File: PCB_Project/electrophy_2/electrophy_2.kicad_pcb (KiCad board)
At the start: 4 copper layers, 35 x 35 mm, 47 parts, among them IC1 ESP32-C3FN4, J1 USB_C_Receptacle_USB2.0_14P, J3 Conn_01x04, U1 LSM6DSV320XTR, U2 BQ21040DBV, U3 TPS27081ADDCR, U4 USBLC6-2SC6, U5 MIC5504-3.3YM5, Y1 40MHZ 15pf, Y2 32 KHz

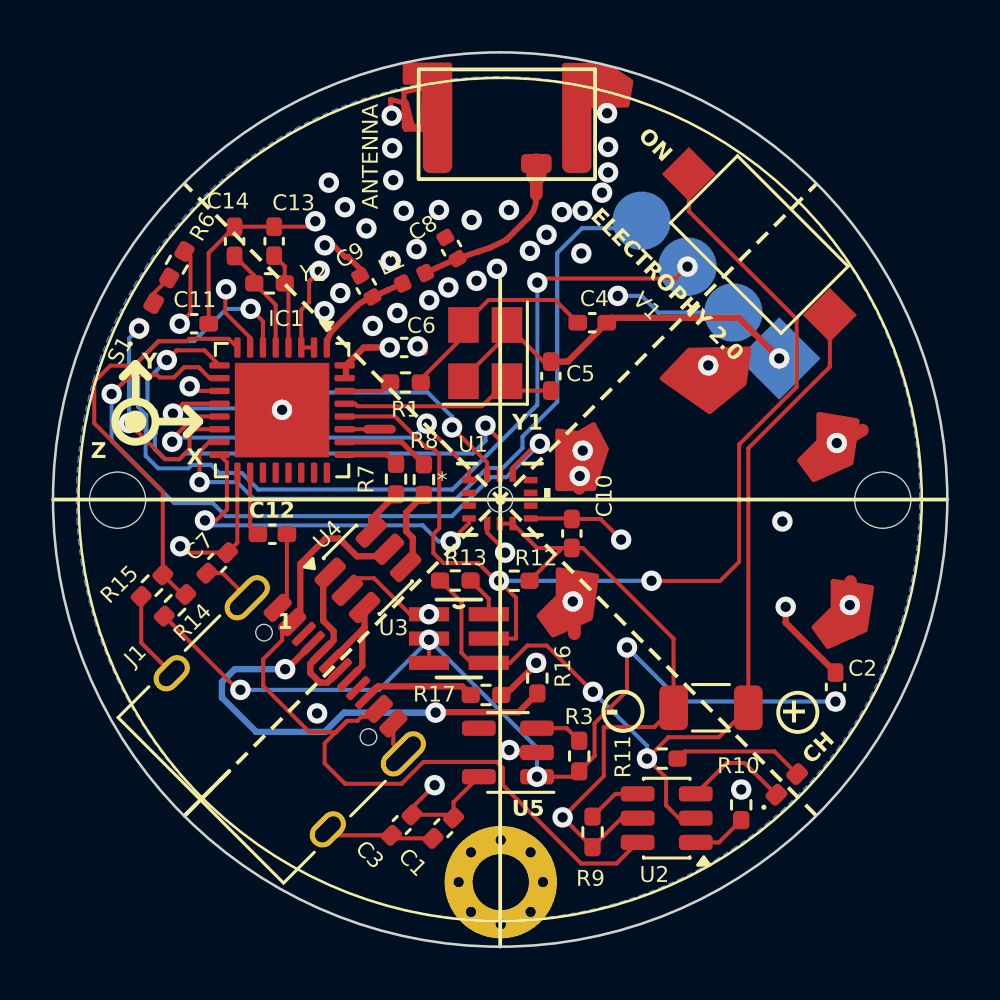
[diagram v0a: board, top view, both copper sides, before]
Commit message: order placed for ElectroPhy 2.0 V1 PCB
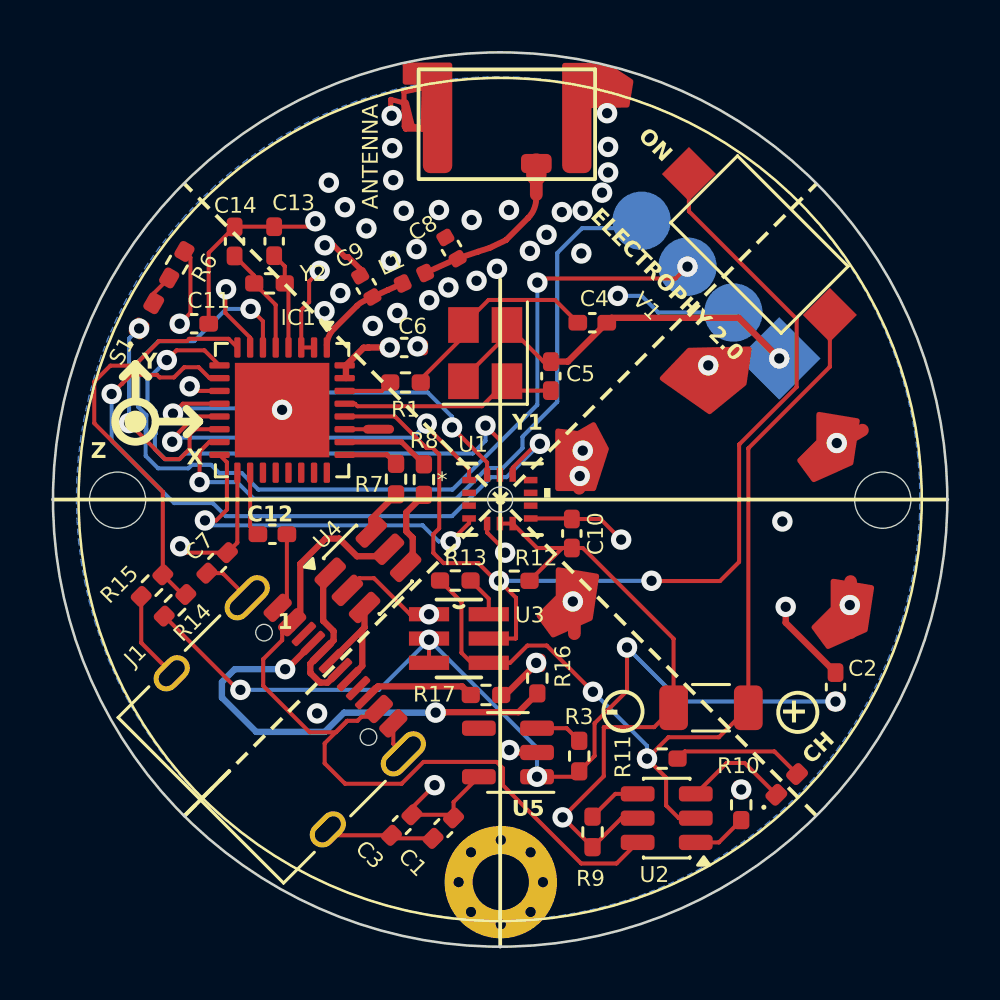
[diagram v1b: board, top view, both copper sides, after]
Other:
- rule pad_to_mask_clearance: 0.08 -> 0
- board text removed: "Notes: OLED display pin pads under the PCB"
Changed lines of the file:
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@@
 			(dielectric_constraints yes)
 		)
-		(pad_to_mask_clearance 0.08)
-		(solder_mask_min_width 0.1524)
+		(pad_to_mask_clearance 0)
 		(allow_soldermask_bridges_in_footprints no)
 		(tenting
@@
 		(tags "resistor handsolder")
 		(property "Reference" "R6"
-			(at 1.795378 0.129686 60)
+			(at 0.441077 1.003968 60)
 			(layer "F.SilkS")
 			(effects
@@
 		(tags "capacitor handsolder")
 		(property "Reference" "C12"
-			(at -0.02 -0.94 0)
+			(at -0.09 -0.79 0)
 			(layer "F.SilkS")
 			(effects
@@
 		(tags "resistor handsolder")
 		(property "Reference" "R7"
-			(at 0 -1.17 90)
+			(at -0.21 -1.06 180)
 			(layer "F.SilkS")
 			(effects
@@
 		(tags "capacitor handsolder")
 		(property "Reference" "C10"
-			(at -1.47 -1.27 90)
+			(at 0.01 -0.93 90)
 			(layer "F.SilkS")
 			(effects
@@
 		(tags "capacitor handsolder")
 		(property "Reference" "C11"
-			(at 0.02 -0.94 0)
+			(at 0.57 -0.91 0)
 			(layer "F.SilkS")
 			(effects
@@
 		(tags "capacitor handsolder")
 		(property "Reference" "C14"
-			(at 1.58 -0.26 180)
+			(at 1.41 0.03 180)
 			(layer "F.SilkS")
 			(effects
@@
 		(tags "TPS27081ADDCR ")
 		(property "Reference" "U3"
-			(at -2.56 -0.42 0)
+			(at 2.77 -0.92 0)
 			(unlocked yes)
 			(layer "F.SilkS")
@@
 		(tags "QFN NoLead")
 		(property "Reference" "IC1"
-			(at -3.58 -0.15 0)
+			(at -3.62 -0.63 0)
 			(layer "F.SilkS")
 			(effects
@@
 		(tags "capacitor handsolder")
 		(property "Reference" "C6"
-			(at 0.67 -0.86 0)
+			(at 0.33 -0.83 0)
 			(layer "F.SilkS")
 			(effects
@@
 			(net "unconnected-(U1-SDX-Pad2)")
 			(pinfunction "SDX_2")
-			(pintype "unspecified")
+			(pintype "unspecified+no_connect")
 		)
 		(pad "3" smd rect
@@
 			(net "unconnected-(U1-SCX-Pad3)")
 			(pinfunction "SCX_3")
-			(pintype "unspecified")
+			(pintype "unspecified+no_connect")
 		)
 		(pad "4" smd rect
@@
 			(net "unconnected-(U1-INT2-Pad9)")
 			(pinfunction "INT2_9")
-			(pintype "unspecified")
+			(pintype "unspecified+no_connect")
 		)
 		(pad "10" smd rect
@@
 			(net "unconnected-(U1-OCS_AUX-Pad10)")
 			(pinfunction "OCS_AUX_10")
-			(pintype "unspecified")
+			(pintype "unspecified+no_connect")
 		)
 		(pad "11" smd rect
@@
 			(net "unconnected-(U1-SDO_AUX-Pad11)")
 			(pinfunction "SDO_AUX_11")
-			(pintype "unspecified")
+			(pintype "unspecified+no_connect")
 		)
 		(pad "12" smd rect
@@
 		(tags "LED handsolder")
 		(property "Reference" "S1"
-			(at -1.684134 -0.217006 60)
+			(at -1.671455 -0.155045 60)
 			(layer "F.SilkS")
 			(effects
@@
 		)
 	)
-	(gr_text "Notes:\nOLED display pin pads under the PCB"
-		(at 183.82 73.64 0)
-		(layer "Cmts.User")
-		(effects
-			(font
-				(size 0.62 0.62)
-				(thickness 0.15)
-				(bold yes)
-			)
-			(justify left bottom)
-		)
-	)
 	(dimension
 		(type aligned)
@@
 	)
 	(segment
+		(start 136.46625 91.98245)
+		(end 137.07125 91.37745)
+		(width 0.16)
+		(layer "F.Cu")
+		(net "Net-(S1-A)")
+	)
+	(segment
+		(start 136.46625 92.3642)
+		(end 136.46625 91.98245)
+		(width 0.16)
+		(layer "F.Cu")
+		(net "Net-(S1-A)")
+	)
+	(segment
 		(start 152.83 100.8125)
 		(end 153.9525 100.8125)
@@
 	)
 	(segment
+		(start 147.5 108.39)
+		(end 147.83 108.39)
+		(width 0.25)
+		(layer "F.Cu")
+		(net "Net-(J1-CC1)")
+	)
+	(segment
+		(start 141.67283 106.69)
+		(end 142.696636 105.666194)
+		(width 0.25)
+		(layer "F.Cu")
+		(net "Net-(J1-CC1)")
+	)
+	(segment
+		(start 147.83 108.39)
+		(end 147.845 108.375)
+		(width 0.25)
+		(layer "F.Cu")
+		(net "Net-(J1-CC1)")
+	)
+	(segment
+		(start 141.61 106.69)
+		(end 141.67283 106.69)
+		(width 0.25)
+		(layer "F.Cu")
+		(net "Net-(J1-CC1)")
+	)
+	(segment
+		(start 150.7425 108.375)
+		(end 151.48 107.6375)
+		(width 0.25)
+		(layer "F.Cu")
+		(net "Net-(J1-CC1)")
+	)
+	(segment
+		(start 147.845 108.375)
+		(end 150.7425 108.375)
+		(width 0.25)
+		(layer "F.Cu")
+		(net "Net-(J1-CC1)")
+	)
+	(via
+		(at 141.61 106.69)
+		(size 0.8)
+		(drill 0.4)
+		(layers "F.Cu" "B.Cu")
+		(net "Net-(J1-CC1)")
+	)
+	(via
+		(at 147.5 108.39)
+		(size 0.8)
+		(drill 0.4)
+		(layers "F.Cu" "B.Cu")
+		(net "Net-(J1-CC1)")
+	)
+	(segment
+		(start 143.160305 109.145)
+		(end 140.479695 109.145)
+		(width 0.25)
+		(layer "B.Cu")
+		(net "Net-(J1-CC1)")
+	)
+	(segment
+		(start 140.479695 109.145)
+		(end 139.135 107.800305)
+		(width 0.25)
+		(layer "B.Cu")
+		(net "Net-(J1-CC1)")
+	)
+	(segment
+		(start 139.135 107.192139)
+		(end 139.637139 106.69)
+		(width 0.25)
+		(layer "B.Cu")
+		(net "Net-(J1-CC1)")
+	)
+	(segment
+		(start 139.135 107.800305)
+		(end 139.135 107.192139)
+		(width 0.25)
+		(layer "B.Cu")
+		(net "Net-(J1-CC1)")
+	)
+	(segment
+		(start 147.5 108.39)
+		(end 143.915305 108.39)
+		(width 0.25)
+		(layer "B.Cu")
+		(net "Net-(J1-CC1)")
+	)
+	(segment
+		(start 139.637139 106.69)
+		(end 141.61 106.69)
+		(width 0.25)
+		(layer "B.Cu")
+		(net "Net-(J1-CC1)")
+	)
+	(segment
+		(start 143.915305 108.39)
+		(end 143.160305 109.145)
+		(width 0.25)
+		(layer "B.Cu")
+		(net "Net-(J1-CC1)")
+	)
+	(segment
 		(start 144.628521 105.148521)
 		(end 144.628521 106.562736)
@@
 	)
 	(segment
+		(start 145.242863 107.362608)
+		(end 144.817957 107.787514)
+		(width 0.25)
+		(layer "F.Cu")
+		(net "Net-(J1-CC2)")
+	)
+	(segment
+		(start 148.535108 107.362608)
+		(end 145.242863 107.362608)
+		(width 0.25)
+		(layer "F.Cu")
+		(net "Net-(J1-CC2)")
+	)
+	(segment
+		(start 148.8725 107.7)
+		(end 148.535108 107.362608)
+		(width 0.25)
+		(layer "F.Cu")
+		(net "Net-(J1-CC2)")
+	)
+	(segment
 		(start 144.439999 96.4)
 		(end 149.31 96.4)
@@
 	(segment
 		(start 144.83 97.3)
-		(end 145.77 97.3)
+		(end 145.7 97.3)
 		(width 0.35)
 		(layer "F.Cu")
@@
 	)
 	(segment
-		(start 158.5875 113.47)
-		(end 157.68 113.47)
-		(width 0.16)
-		(layer "F.Cu")
-		(net "Net-(U2-TS)")
-	)
-	(segment
-		(start 159.46 112.5975)
-		(end 158.5875 113.47)
-		(width 0.16)
-		(layer "F.Cu")
-		(net "Net-(U2-TS)")
-	)
-	(segment
 		(start 157.68 111.57)
 		(end 158.89 110.36)
@@
 	)
 	(segment
-		(start 136.46625 91.98245)
-		(end 137.07125 91.37745)
+		(start 158.5875 113.47)
+		(end 157.68 113.47)
 		(width 0.16)
 		(layer "F.Cu")
-		(net "Net-(S1-A)")
+		(net "Net-(U2-TS)")
 	)
 	(segment
-		(start 136.46625 92.3642)
-		(end 136.46625 91.98245)
+		(start 159.46 112.5975)
+		(end 158.5875 113.47)
 		(width 0.16)
 		(layer "F.Cu")
-		(net "Net-(S1-A)")
-	)
-	(segment
-		(start 145.242863 107.362608)
-		(end 144.817957 107.787514)
-		(width 0.25)
-		(layer "F.Cu")
-		(net "Net-(J1-CC2)")
-	)
-	(segment
-		(start 148.535108 107.362608)
-		(end 145.242863 107.362608)
-		(width 0.25)
-		(layer "F.Cu")
-		(net "Net-(J1-CC2)")
-	)
-	(segment
-		(start 148.8725 107.7)
-		(end 148.535108 107.362608)
-		(width 0.25)
-		(layer "F.Cu")
-		(net "Net-(J1-CC2)")
-	)
-	(segment
-		(start 147.5 108.39)
-		(end 147.83 108.39)
-		(width 0.25)
-		(layer "F.Cu")
-		(net "Net-(J1-CC1)")
-	)
-	(segment
-		(start 141.67283 106.69)
-		(end 142.696636 105.666194)
-		(width 0.25)
-		(layer "F.Cu")
-		(net "Net-(J1-CC1)")
-	)
-	(segment
-		(start 147.83 108.39)
-		(end 147.845 108.375)
-		(width 0.25)
-		(layer "F.Cu")
-		(net "Net-(J1-CC1)")
-	)
-	(segment
-		(start 141.61 106.69)
-		(end 141.67283 106.69)
-		(width 0.25)
-		(layer "F.Cu")
-		(net "Net-(J1-CC1)")
-	)
-	(segment
-		(start 150.7425 108.375)
-		(end 151.48 107.6375)
-		(width 0.25)
-		(layer "F.Cu")
-		(net "Net-(J1-CC1)")
-	)
-	(segment
-		(start 147.845 108.375)
-		(end 150.7425 108.375)
-		(width 0.25)
-		(layer "F.Cu")
-		(net "Net-(J1-CC1)")
-	)
-	(via
-		(at 141.61 106.69)
-		(size 0.8)
-		(drill 0.4)
-		(layers "F.Cu" "B.Cu")
-		(net "Net-(J1-CC1)")
-	)
-	(via
-		(at 147.5 108.39)
-		(size 0.8)
-		(drill 0.4)
-		(layers "F.Cu" "B.Cu")
-		(net "Net-(J1-CC1)")
-	)
-	(segment
-		(start 143.160305 109.145)
-		(end 140.479695 109.145)
-		(width 0.25)
-		(layer "B.Cu")
-		(net "Net-(J1-CC1)")
-	)
-	(segment
-		(start 140.479695 109.145)
-		(end 139.135 107.800305)
-		(width 0.25)
-		(layer "B.Cu")
-		(net "Net-(J1-CC1)")
-	)
-	(segment
-		(start 139.135 107.192139)
-		(end 139.637139 106.69)
-		(width 0.25)
-		(layer "B.Cu")
-		(net "Net-(J1-CC1)")
-	)
-	(segment
-		(start 139.135 107.800305)
-		(end 139.135 107.192139)
-		(width 0.25)
-		(layer "B.Cu")
-		(net "Net-(J1-CC1)")
-	)
-	(segment
-		(start 147.5 108.39)
-		(end 143.915305 108.39)
-		(width 0.25)
-		(layer "B.Cu")
-		(net "Net-(J1-CC1)")
-	)
-	(segment
-		(start 139.637139 106.69)
-		(end 141.61 106.69)
-		(width 0.25)
-		(layer "B.Cu")
-		(net "Net-(J1-CC1)")
-	)
-	(segment
-		(start 143.915305 108.39)
-		(end 143.160305 109.145)
-		(width 0.25)
-		(layer "B.Cu")
-		(net "Net-(J1-CC1)")
+		(net "Net-(U2-TS)")
 	)
 	(zone
